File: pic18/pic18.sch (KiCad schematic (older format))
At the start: 90 parts, among them J1 PORTA, J10 PORTE, J11 5v-3.3v, J12 5v-3.3v, J14 PICKIT3, J15 CONTROL, J2 PORTB, J20 LED'S, J21 BUZZER, J3 Barrel_Jack_Switch, J4 Vin, J5 TECLADO, J6 OLED, J7 PORTD, J8 HC-05, J9 PORTC, SW1 SW_Push, SW2 SW_DIP_x01, U1 PIC18F45K50, U2 3x7Segment, U3 NRF24L01_Breakout, U4 AMS1117-5.0, U5 AMS1117-3.3

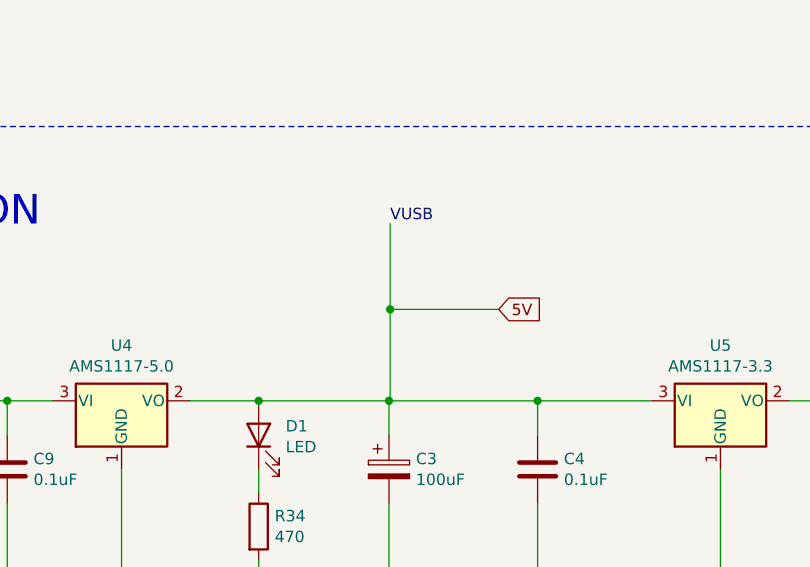
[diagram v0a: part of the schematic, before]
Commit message: JaPic
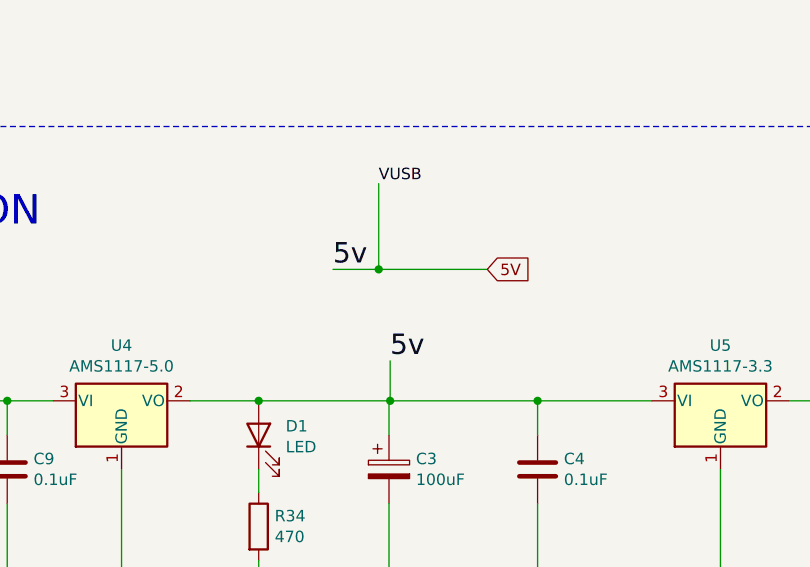
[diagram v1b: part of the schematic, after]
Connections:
- net 5V: now also C4.1, D1.2 (A), U4.2 (VO), U5.3 (VI)
- now unconnected: C3.1
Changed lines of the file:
@@
 	3100 6500 3400 6500
 Connection ~ 3400 6500
-Wire Wire Line
-	3400 6500 3970 6500
-Connection ~ 3970 6500
-Wire Wire Line
-	3970 6500 4620 6500
-Wire Wire Line
-	3975 5725 3975 6100
-Wire Wire Line
-	3975 6100 4450 6100
-Connection ~ 3975 6100
-Wire Wire Line
-	3975 6100 3975 6500
-Text GLabel 4450 6100 2    50   Input ~ 0
-5V
-Text Label 3975 5725 0    50   ~ 0
+Text Label 3925 5550 0    50   ~ 0
 VUSB
 $Comp
@@
 Text Label 11300 6250 0    50   ~ 0
 GND1
+Wire Wire Line
+	3925 5550 3925 5925
+Wire Wire Line
+	3925 5925 4400 5925
+Text GLabel 4400 5925 2    50   Input ~ 0
+5V
+Wire Wire Line
+	3400 6500 3975 6500
+Wire Wire Line
+	3975 6500 3975 6325
+Connection ~ 3975 6500
+Wire Wire Line
+	3975 6500 4620 6500
+Text Label 3975 6325 0    89   ~ 0
+5v
+Wire Wire Line
+	3925 5925 3725 5925
+Connection ~ 3925 5925
+Text Label 3725 5925 0    89   ~ 0
+5v
 $EndSCHEMATC

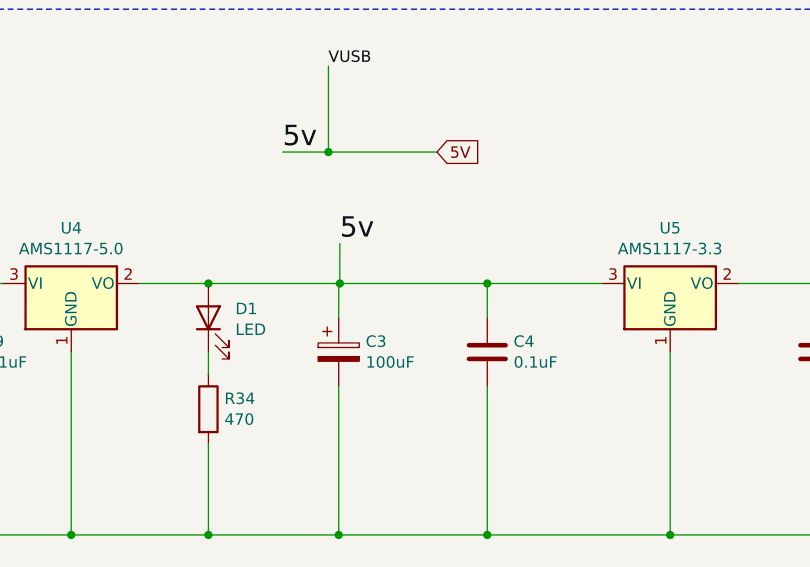
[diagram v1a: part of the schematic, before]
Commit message: JaPic
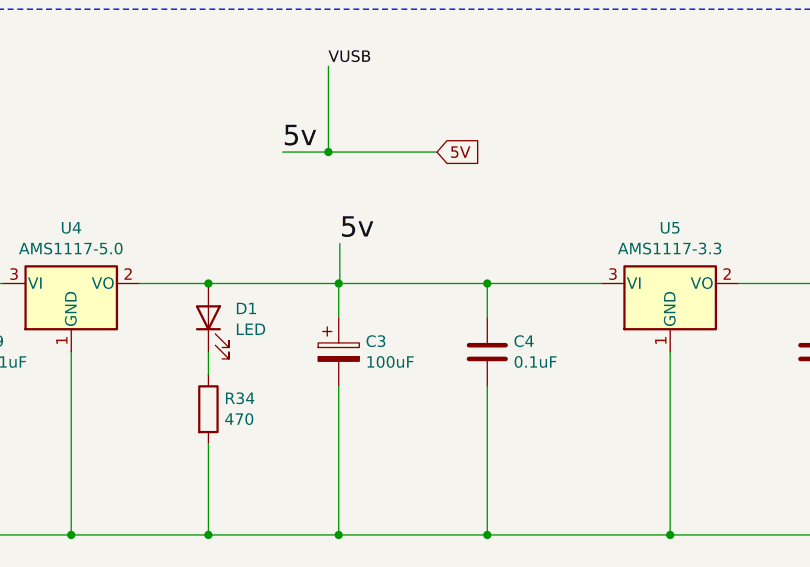
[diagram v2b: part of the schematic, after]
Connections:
- net 5V: now also C3.1
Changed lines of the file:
@@
 	1    0    0    -1
 $EndComp
-Connection ~ 4620 6500
-Wire Wire Line
-	5120 6500 4620 6500
 Wire Wire Line
 	4620 6650 4620 6500
@@
 Wire Wire Line
 	3100 6500 3400 6500
-Connection ~ 3400 6500
 Text Label 3925 5550 0    50   ~ 0
 VUSB
@@
 5V
 Wire Wire Line
-	3400 6500 3975 6500
-Wire Wire Line
 	3975 6500 3975 6325
-Connection ~ 3975 6500
-Wire Wire Line
-	3975 6500 4620 6500
 Text Label 3975 6325 0    89   ~ 0
 5v
@@
 Text Label 3725 5925 0    89   ~ 0
 5v
+Wire Wire Line
+	3975 6500 3970 6500
+Connection ~ 3400 6500
+Connection ~ 3970 6500
+Wire Wire Line
+	3970 6500 3400 6500
+Wire Wire Line
+	3975 6500 4620 6500
+Connection ~ 4620 6500
+Wire Wire Line
+	4620 6500 5120 6500
 $EndSCHEMATC
